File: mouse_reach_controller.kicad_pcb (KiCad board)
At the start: 2 copper layers, 0 parts

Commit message: Initial layout
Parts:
- added C1: 0.1uF, mouse_reach_controller:SM0402, F.Cu at (157.5, 101.6)
- added C10: 0.1uF, mouse_reach_controller:SM0402, F.Cu at (115.6, 90.2)
- added C11: 2.2uF, mouse_reach_controller:SM0402, F.Cu at (102.9, 90.2)
- added C12: 0.1uF, mouse_reach_controller:SM0402, F.Cu at (102.9, 92.7)
- added C13: 2.2uF, mouse_reach_controller:SM0402, F.Cu at (125.1, 99.1)
- added C14: 0.1uF, mouse_reach_controller:SM0402, F.Cu at (122.6, 99.1)
- added C15: 2.2uF, mouse_reach_controller:SM0402, F.Cu at (116.2, 99.1)
- added C16: 0.15uF, mouse_reach_controller:SM0402, F.Cu at (102.9, 99.1)
- added C2: 0.1uF, mouse_reach_controller:SM0402, F.Cu at (175.3, 96.5)
- added C3: 0.1uF, mouse_reach_controller:SM0402, F.Cu at (137.2, 66.0)
- added C4: 0.1uF, mouse_reach_controller:SM0402, F.Cu at (74.3, 61.6)
- added C5: 0.1uF, mouse_reach_controller:SM0402, F.Cu at (170.2, 66.0)
- added C6: 0.1uF, mouse_reach_controller:SM0402, F.Cu at (95.9, 81.9)
- added C7: 0.1uF, mouse_reach_controller:SM0402, F.Cu at (203.2, 66.0)
- added C8: 0.1uF, mouse_reach_controller:SM0402, F.Cu at (95.9, 76.8)
- added C9: 2.2uF, mouse_reach_controller:SM0402, F.Cu at (102.2, 71.8)
- added CLK1: CLK_32MHZ, mouse_reach_controller:CTS_SMD_4_7X5MM, F.Cu at (157.5, 96.5)
- added D1: DIODE_SCHOTTKY_30V_200mA_0402, mouse_reach_controller:SM0402_POL, F.Cu at (102.2, 65.4)
- added FID1: FIDUCIAL, mouse_reach_controller:FIDUCIAL, F.Cu at (72.4, 61.0)
- added FID2: FIDUCIAL, mouse_reach_controller:FIDUCIAL, F.Cu at (224.8, 61.0)
- added FID3: FIDUCIAL, mouse_reach_controller:FIDUCIAL, F.Cu at (224.8, 99.1)
- added FID4: FIDUCIAL, mouse_reach_controller:FIDUCIAL, F.Cu at (72.4, 99.1)
- added J1: AUDIO_JACK_3.5MM, mouse_reach_controller:AUDIO_JACK_3.5MM_3PIN, F.Cu at (114.3, 53.3)
- added L1: 600@100MHz_1210, mouse_reach_controller:SM1210, F.Cu at (109.2, 90.2)
- added MH1: MOUNTING_HOLE_4-40, mouse_reach_controller:MOUNTING_HOLE_4-40, F.Cu at (72.4, 54.6)
- added MH2: MOUNTING_HOLE_4-40, mouse_reach_controller:MOUNTING_HOLE_4-40, F.Cu at (224.8, 54.6)
- added MH3: MOUNTING_HOLE_4-40, mouse_reach_controller:MOUNTING_HOLE_4-40, F.Cu at (224.8, 105.4)
- added MH4: MOUNTING_HOLE_4-40, mouse_reach_controller:MOUNTING_HOLE_4-40, F.Cu at (72.4, 105.4)
- added P1: HEADER_02X05_LATCH, mouse_reach_controller:HEADER_02x05_LATCH, F.Cu at (137.2, 58.4)
- added P2: HEADER_02X05_LATCH, mouse_reach_controller:HEADER_02x05_LATCH, F.Cu at (170.2, 58.4)
- added P3: HEADER_02X05_LATCH, mouse_reach_controller:HEADER_02x05_LATCH, F.Cu at (203.2, 58.4)
- added R1: 100, mouse_reach_controller:SM0402, F.Cu at (132.1, 68.6)
- added R2: 100, mouse_reach_controller:SM0402, F.Cu at (132.1, 74.9)
- added R3: 100, mouse_reach_controller:SM0402, F.Cu at (165.1, 68.6)
- added R4: 100, mouse_reach_controller:SM0402, F.Cu at (165.1, 74.9)
- added R5: 100, mouse_reach_controller:SM0402, F.Cu at (198.1, 68.6)
- added R6: 100, mouse_reach_controller:SM0402, F.Cu at (198.1, 74.9)
- added R7: 2.21k, mouse_reach_controller:SM0402, F.Cu at (95.9, 74.3)
- added R8: 2.21k, mouse_reach_controller:SM0402, F.Cu at (95.9, 71.8)
- added T1: TERM_BLK_HDR_2POS_90DEG_0.2IN, mouse_reach_controller:TERM_BLK_HDR_2POS_90DEG_0.2IN, F.Cu at (102.2, 62.2)
- added TEENSY1: TEENSY_4.0_PIN_RECEPTACLES, mouse_reach_controller:TEENSY_4.0_PIN_RECEPTACLES, F.Cu at (85.1, 70.5)
- added U1: TMC429, mouse_reach_controller:QFN-32-1EP_5x5mm_P0.5mm_EP3.3x3.3mm, F.Cu at (170.2, 96.5)
- added U10: SGTL5000, mouse_reach_controller:QFN-32-1EP_5x5mm_P0.5mm_EP3.3x3.3mm, F.Cu at (109.2, 99.1)
- added U2: SN65LVDM050QDRQ1, mouse_reach_controller:SOIC_16_0.154IN, F.Cu at (137.2, 72.4)
- added U3: BUFFER_TRI_STATE_SMALL, mouse_reach_controller:MICROPAK2_6LEAD, F.Cu at (74.3, 59.1)
- added U4: SN65LVDM050QDRQ1, mouse_reach_controller:SOIC_16_0.154IN, F.Cu at (170.2, 72.4)
- added U5: BUFFER_TRI_STATE_SMALL, mouse_reach_controller:MICROPAK2_6LEAD, F.Cu at (95.9, 84.5)
- added U6: SN65LVDM050QDRQ1, mouse_reach_controller:SOIC_16_0.154IN, F.Cu at (203.2, 72.4)
- added U7: BUFFER_TRI_STATE_SMALL, mouse_reach_controller:MICROPAK2_6LEAD, F.Cu at (95.9, 79.4)
- added U8: MIC94091YC6-TR, mouse_reach_controller:SC70-6, F.Cu at (102.2, 68.6)
- added U9: RT9076-15GV, mouse_reach_controller:SOT-23-3, F.Cu at (119.4, 99.1)
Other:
- board outline added: 157.5 x 55.9 mm
- net class Default: clearance 0.2 -> 0.1016; trace_width 0.25 -> 0.4064; via_dia 0.8 -> 0.889; via_drill 0.4 -> 0.635
- rule trace_clearance: 0.2 -> 0.1016

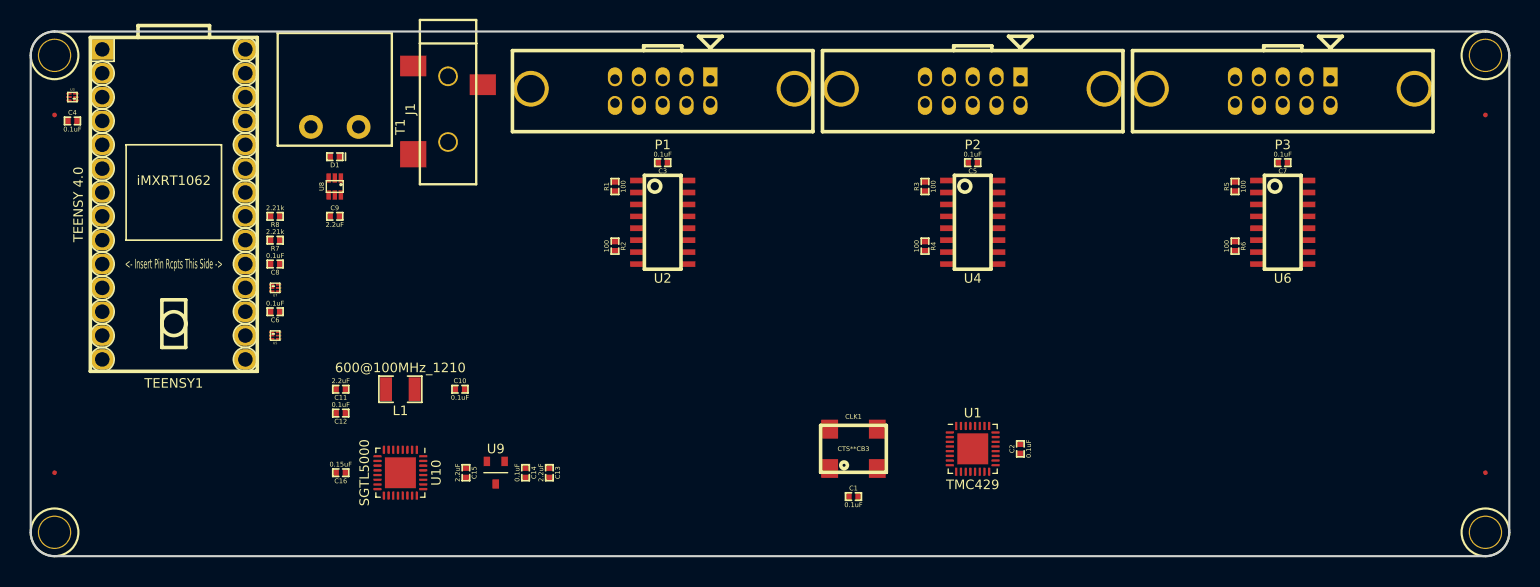
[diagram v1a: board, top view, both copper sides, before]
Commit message: Finish layout
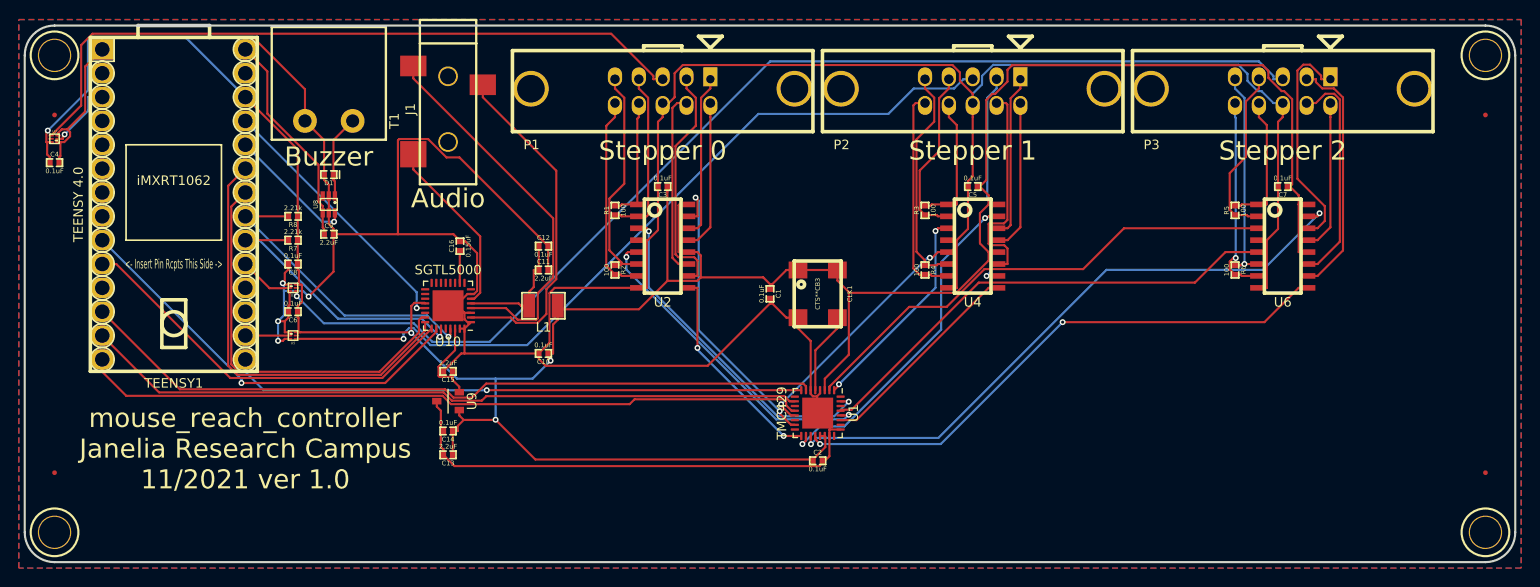
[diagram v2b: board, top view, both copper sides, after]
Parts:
- moved C12 28.0 mm to (124.5, 74.9), turned to 90 degrees
- moved C16 27.3 mm to (115.6, 74.9), turned to 180 degrees
- moved C11 25.0 mm to (124.5, 77.5), turned to 90 degrees
- moved C1 23.3 mm to (148.6, 80.0), turned to 0 degrees
- moved C2 21.6 mm to (153.7, 97.8), turned to 90 degrees
- moved U10 18.5 mm to (114.3, 81.3), turned to 180 degrees
- moved L1 17.6 mm to (124.5, 81.3)
- moved U1 16.9 mm to (153.7, 92.7), turned to 270 degrees
- moved CLK1 16.9 mm to (153.7, 80.0), turned to 270 degrees
- moved C13 11.0 mm to (114.3, 97.2), turned to 270 degrees
- moved C15 11.0 mm to (114.3, 88.3), turned to 270 degrees
- moved C10 9.67 mm to (124.5, 86.4), turned to 270 degrees
- moved C14 9.38 mm to (114.3, 94.6), turned to 270 degrees
- moved U9 9.16 mm to (114.3, 91.4), turned to 90 degrees
- moved C4 4.84 mm to (72.4, 66.0)
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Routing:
- net /GND: track 0.00 -> 421.3 mm, vias 0 -> 4
- net /VDD: track 0.00 -> 318.1 mm, vias 0 -> 4
- net /stepper_controller/stepper_driver_interface_2/UART_BUFFERED: track 0.00 -> 120.9 mm, vias 0 -> 1
- net /stepper_controller/stepper_driver_interface_1/UART_BUFFERED: track 0.00 -> 85.3 mm, vias 0 -> 1
- net /~CS: track 0.00 -> 79.9 mm
- net /MISO: track 0.00 -> 77.4 mm
- net /MOSI: track 0.00 -> 77.1 mm
- net /stepper_controller/stepper_driver_interface_0/UART_BUFFERED: track 0.00 -> 75.6 mm
- net /stepper_controller/STEP_2: track 0.00 -> 66.7 mm, vias 0 -> 2
- net /SCK: track 0.00 -> 61.3 mm, vias 0 -> 1
- net /stepper_controller/DIR_2: track 0.00 -> 59.9 mm, vias 0 -> 2
- net /stepper_controller/REF_2: track 0.00 -> 52.9 mm
- net /stepper_controller/REFR_2: track 0.00 -> 51.4 mm
- net /BCLK: track 0.00 -> 46.0 mm
- net /I2S_DIN: track 0.00 -> 44.7 mm, vias 0 -> 1
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- added copper zone on B.Cu, net /GND
- added copper zone on F.Cu, net /GND
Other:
- board size 157.5 x 55.9 mm -> 158.8 x 57.2 mm
- net class Default: trace_width 0.4064 -> 0.2286; via_dia 0.889 -> 0.635; via_drill 0.635 -> 0.4064
- net class GROUND added: clearance 0.1016, trace_width 0.2286, via_dia 0.635, via_drill 0.4064
- net class POWER: trace_width 0.4064 -> 0.2286; via_dia 0.889 -> 0.635; via_drill 0.635 -> 0.4064
- net class SENSE added: clearance 0.1016, trace_width 0.2286, via_dia 0.635, via_drill 0.4064
- net class SIGNAL added: clearance 0.1016, trace_width 0.2286, via_dia 0.635, via_drill 0.4064
- net class THICKPOWER added: clearance 0.2032, trace_width 1.524, via_dia 1.524, via_drill 0.635
- net class THICKSIGNAL added: clearance 0.2032, trace_width 0.6096, via_dia 0.9144, via_drill 0.635
- rule trace_min: 0.2 -> 0.127
- board text added: "Audio"
- board text added: "Buzzer"
- board text added: "Stepper 0"
- board text added: "Stepper 1"
- board text added: "Stepper 2"
- board text added: "mouse_reach_controller Janelia Research Campus 11/2021 ver 1.0"
